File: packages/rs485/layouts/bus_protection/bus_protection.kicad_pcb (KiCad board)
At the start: 2 copper layers, 10 parts

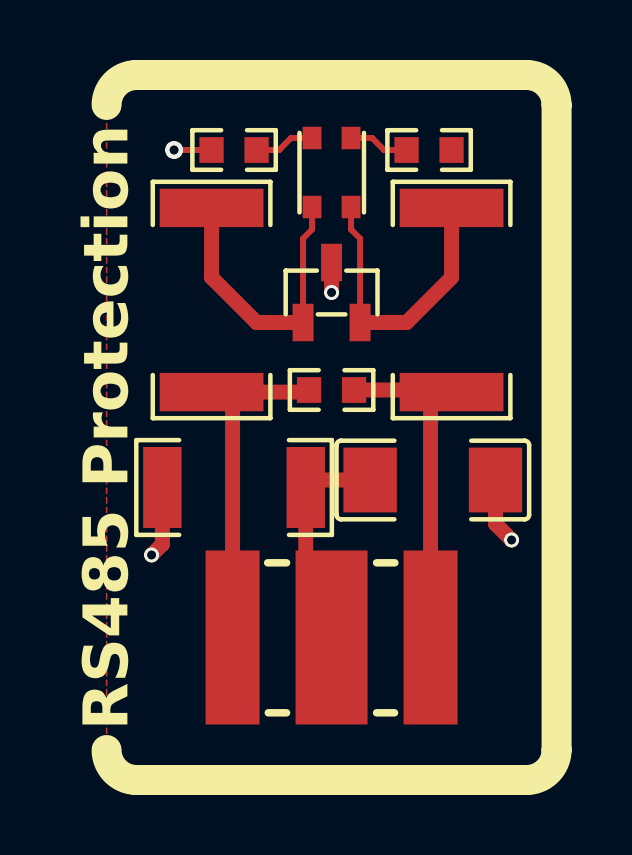
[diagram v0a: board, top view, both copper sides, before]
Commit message: Rebuild all
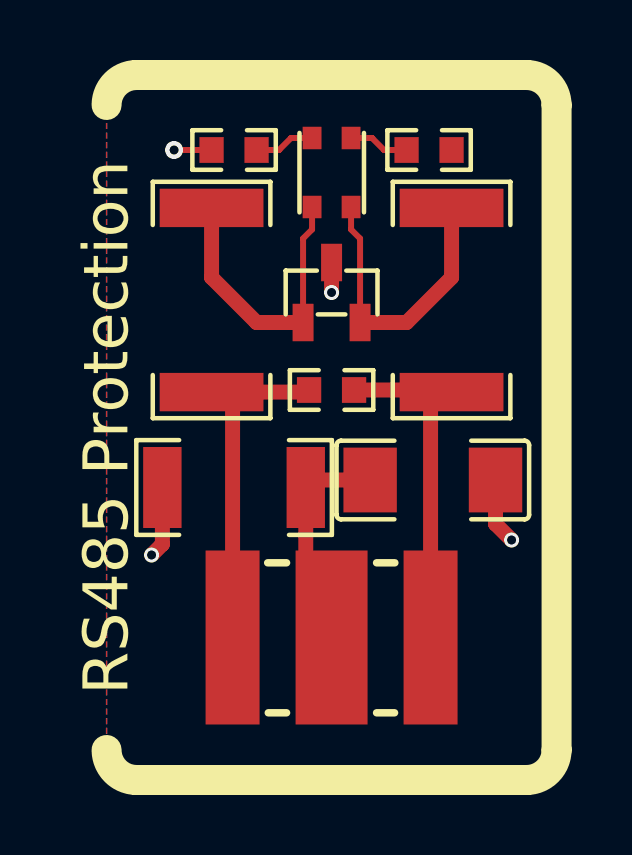
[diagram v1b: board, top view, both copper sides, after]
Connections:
- FL1 pad 1: line-2 -> line-1
- FL1 pad 2: line -> line-3
- FL1 pad 3: line-3 -> line
- FL1 pad 4: line-1 -> line-2
- R1 pad 1: line -> line-3
- R2 pad 1: line-2 -> line-1
- R4 pad 1: line-3 -> line
- R5 pad 1: line-1 -> line-2
- U1 pad 1: line-2 -> line-1
- U1 pad 2: line -> line-3
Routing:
- net line-3: track 2.02 -> 9.97 mm
- net line-2: track 9.97 -> 2.02 mm
- net line-1: track 2.02 -> 9.97 mm
- net line: track 9.97 -> 2.02 mm
